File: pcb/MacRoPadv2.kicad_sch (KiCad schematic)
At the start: 15 parts, among them J1 Conn_01x04, SW1 SW_Push, SW2 SW_Push, SW3 SW_Push, SW4 SW_Push, SW5 SW_Push, SW6 SW_Push, SW7 RotaryEncoder, SW8 RotaryEncoder, U1 MOUDLE-SEEEDUINO-XIAO

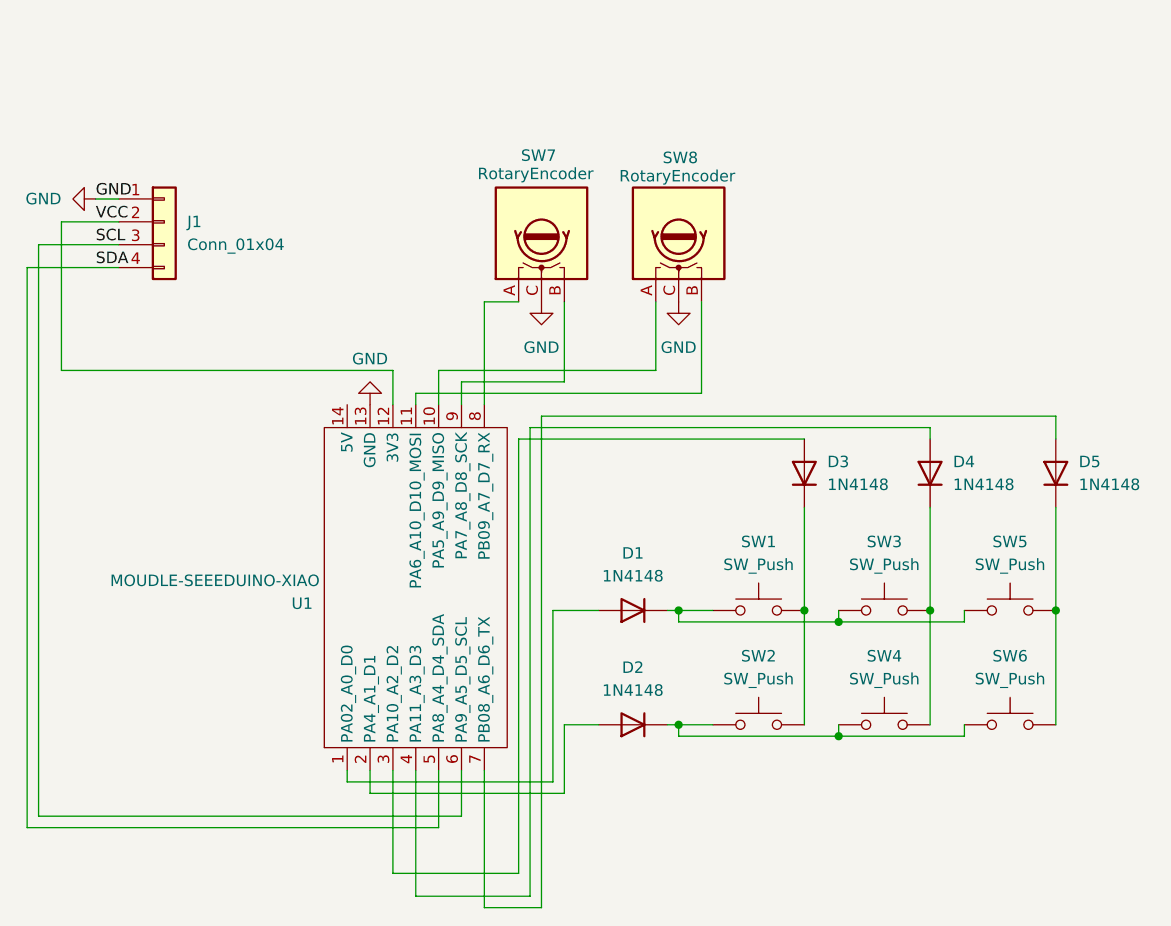
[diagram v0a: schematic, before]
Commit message: Add files via upload
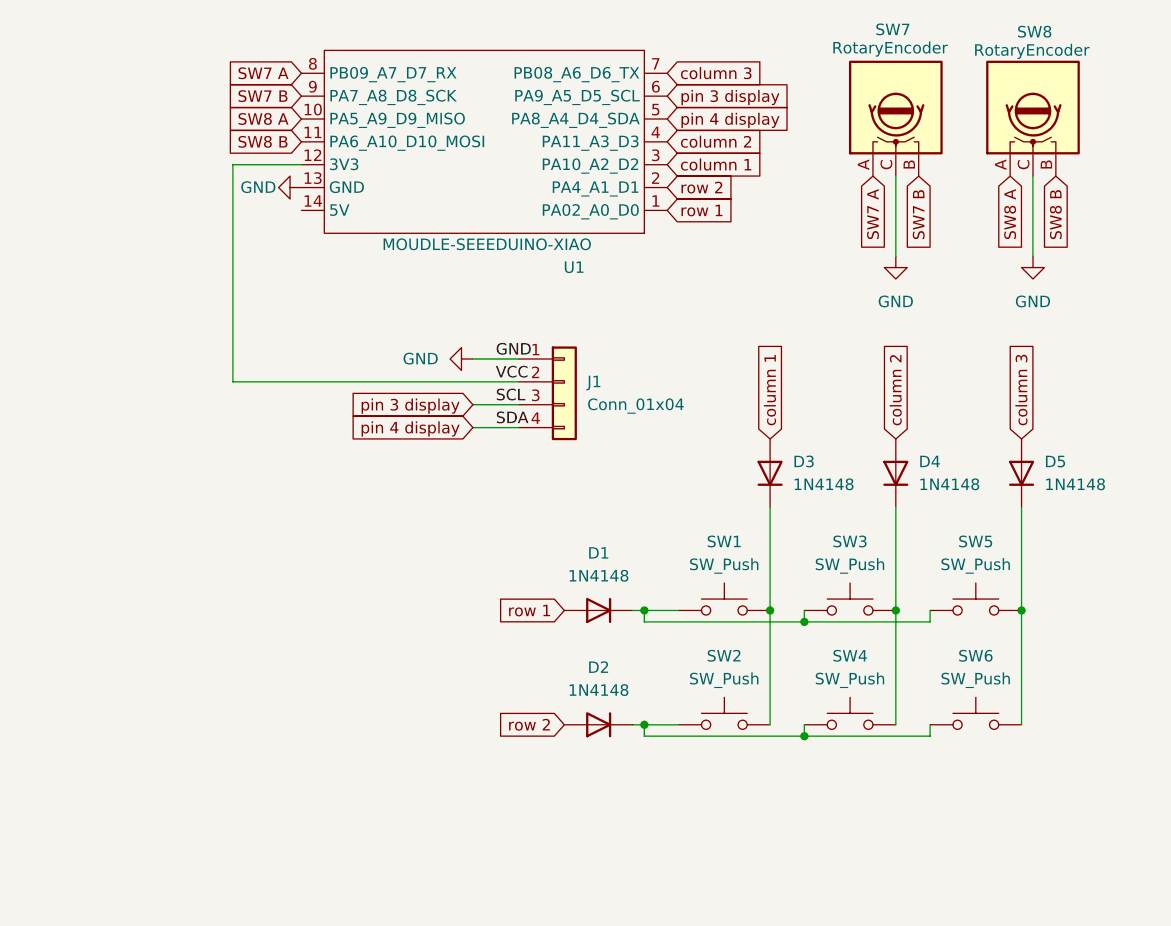
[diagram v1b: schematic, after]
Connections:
- net row 1: now reaches D1.2 (A), U1.1 (PA02_A0_D0)
- net SW8 A: now reaches SW8.A, U1.10 (PA5_A9_D9_MISO)
- net SW8 B: now reaches SW8.B, U1.11 (PA6_A10_D10_MOSI)
- net row 2: now reaches D2.2 (A), U1.2 (PA4_A1_D1)
- net column 1: now reaches D3.2 (A), U1.3 (PA10_A2_D2)
- net column 2: now reaches D4.2 (A), U1.4 (PA11_A3_D3)
- net column 3: now reaches D5.2 (A), U1.7 (PB08_A6_D6_TX)
- net SW7 A: now reaches SW7.A, U1.8 (PB09_A7_D7_RX)
- net SW7 B: now reaches SW7.B, U1.9 (PA7_A8_D8_SCK)
- net SCL renamed pin 3 display
- net SDA renamed pin 4 display
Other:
- moved on the sheet: D1, D2, D3, D4, D5, J1, SW1, SW2, SW3, SW4, SW5, SW6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

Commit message: Add files via upload
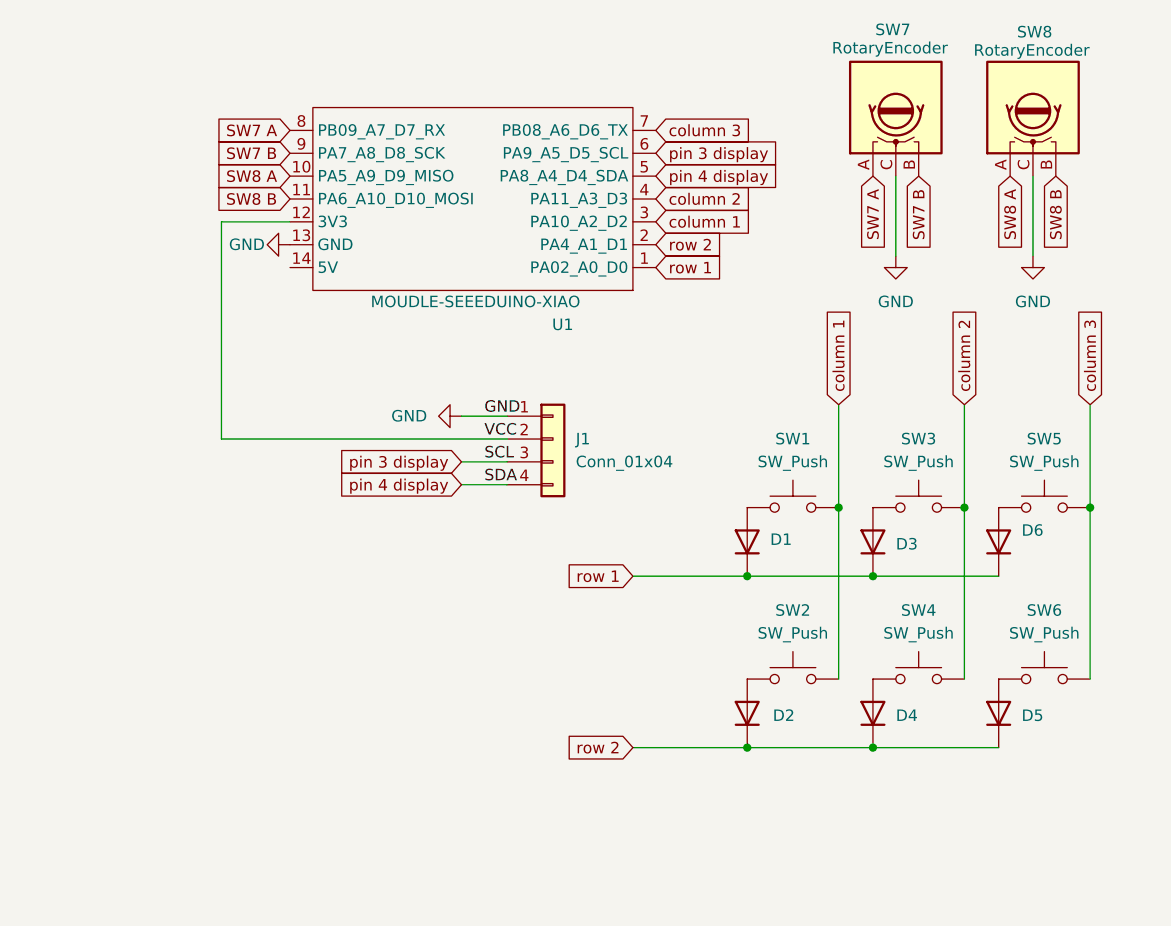
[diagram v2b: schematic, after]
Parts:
- added D6: 1N4148, Diode_THT:D_DO-35_SOD27_P7.62mm_Horizontal, symbol Diode:1N4148
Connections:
- net column 1: now also SW1.2, SW2.2; no longer D3.2 (A)
- net column 2: now also SW3.2, SW4.2; no longer D4.2 (A)
- net column 3: now also SW5.2, SW6.2; no longer D5.2 (A)
- net row 1: now also D1.1 (K), D3.1 (K), D6.1 (K); no longer D1.2 (A)
- net row 2: now also D2.1 (K), D4.1 (K), D5.1 (K); no longer D2.2 (A)
- new net: D2.2 (A), SW2.1
- new net: D6.2 (A), SW5.1
- new net: D5.2 (A), SW6.1
- new net: D4.2 (A), SW4.1
- new net: D1.2 (A), SW1.1
- new net: D3.2 (A), SW3.1
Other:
- moved on the sheet: D1, D2, D3, D4, D5, J1, SW1, SW2, SW3, SW4, SW5, SW6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
